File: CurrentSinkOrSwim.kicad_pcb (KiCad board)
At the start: 2 copper layers, 41.7 x 47.8 mm, 22 parts, among them P1 HEATSINK, P101 CONN_01X02, P102 CONN_01X03, P103 CONN_01X02, Q401 BUK9575, U201 LMV358, U301 LM2931

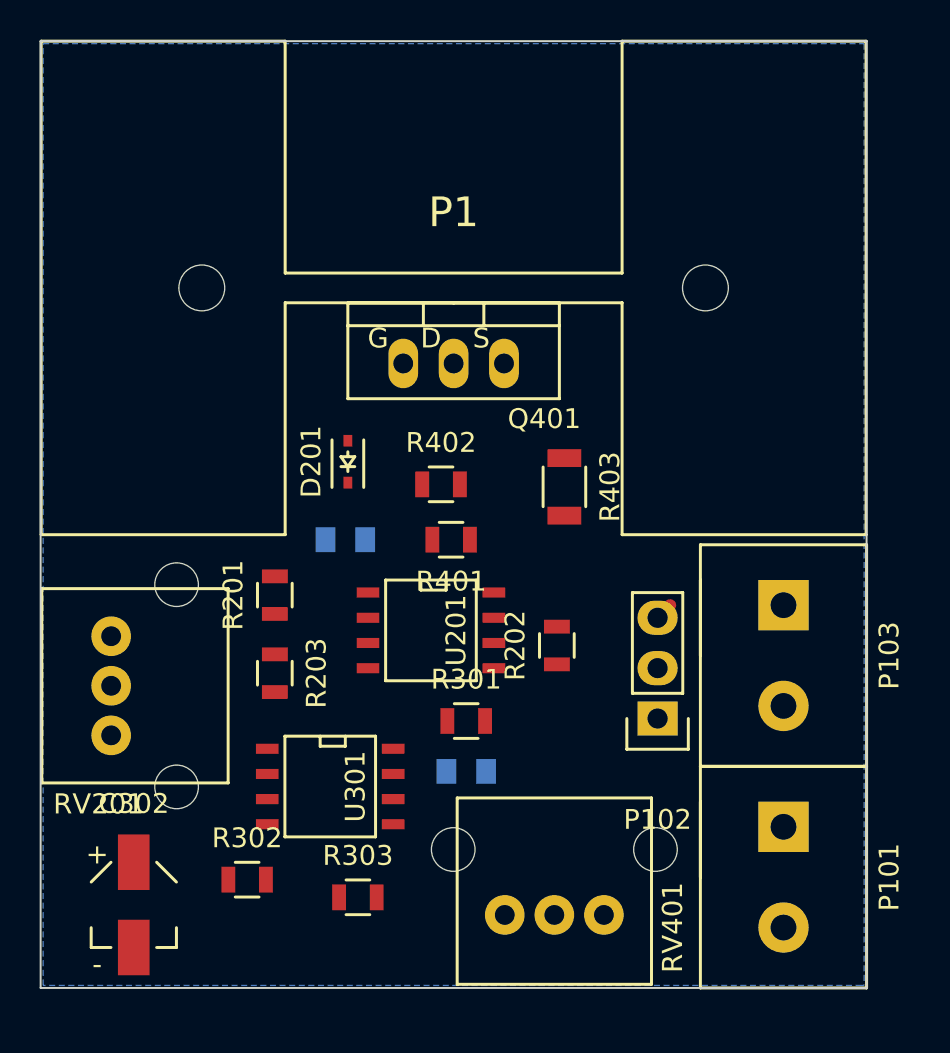
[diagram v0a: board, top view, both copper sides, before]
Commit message: possible layout with over half of tracks
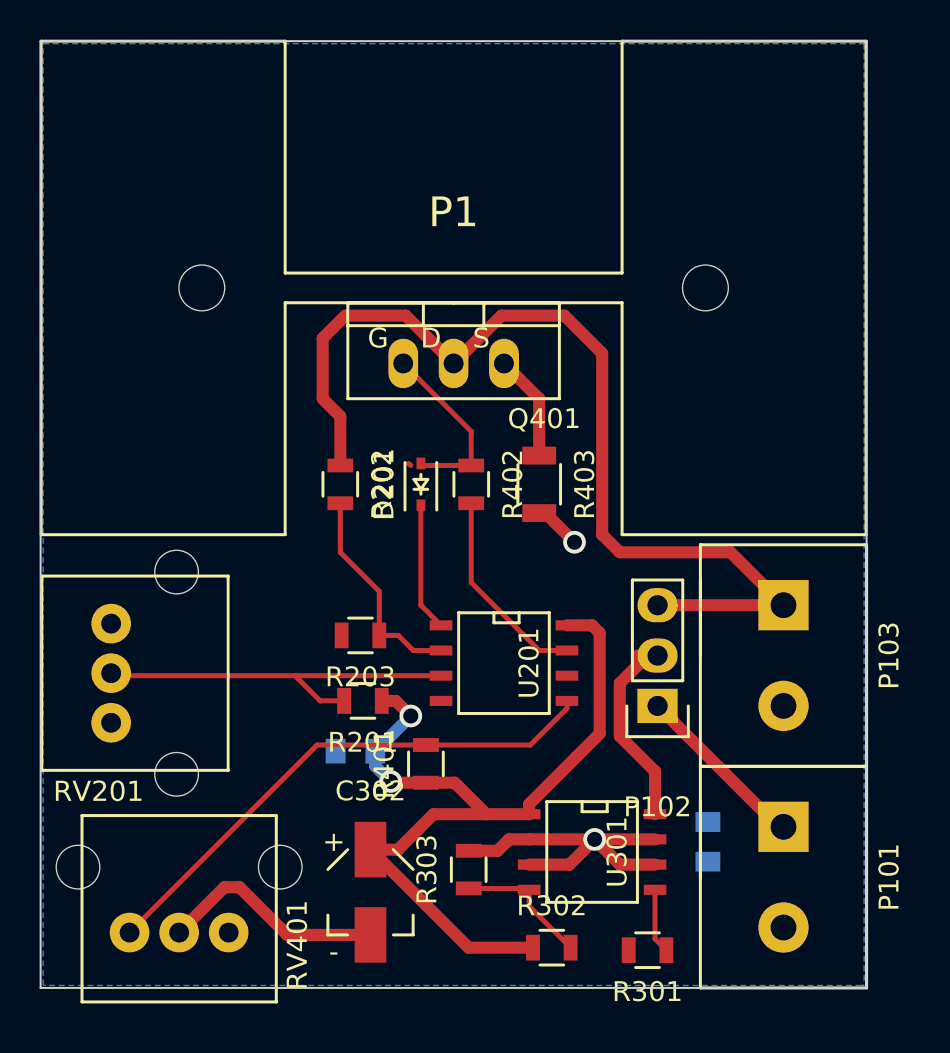
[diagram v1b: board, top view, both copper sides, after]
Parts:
- moved RV401 18.9 mm to (113.2, 80.8)
- moved R302 15.7 mm to (132.0, 81.5)
- moved R301 14.7 mm to (136.8, 81.7), turned to 180 degrees
- moved U301 13.6 mm to (134.0, 76.7)
- moved R202 13.6 mm to (121.3, 58.2), turned to 270 degrees
- moved C301 12.7 mm to (139.8, 76.2), turned to 270 degrees
- moved C302 12.0 mm to (122.8, 78.7)
- moved R401 11.4 mm to (125.6, 72.3), turned to 90 degrees
- moved C201 10.7 mm to (122.0, 71.6), turned to 180 degrees
- moved R201 6.94 mm to (122.4, 69.1), turned to 180 degrees
- moved R303 5.76 mm to (127.8, 77.6), turned to 90 degrees
- moved R203 4.72 mm to (122.3, 65.8), turned to 180 degrees
- moved U201 4.04 mm to (129.5, 67.2)
- moved D201 3.86 mm to (125.3, 58.2)
- moved R402 1.52 mm to (127.9, 58.2), turned to 270 degrees
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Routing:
- net /Current Control/Current_Sink+: track 1.66 -> 50.3 mm
- net 2.7V: track 0.00 -> 43.1 mm, vias 0 -> 2
- net GND: track 0.00 -> 31.1 mm, vias 0 -> 2
- net Net-(R401-Pad2): track 0.00 -> 27.2 mm
- net Net-(R201-Pad2): track 0.00 -> 19.7 mm
- net Net-(R202-Pad2): track 0.00 -> 10.9 mm
- net /Power Regulation/Vin: track 0.00 -> 10.8 mm
- net Net-(R402-Pad2): track 0.00 -> 10.2 mm
- net /Current Control/FET_Gate: track 0.00 -> 9.69 mm
- net Net-(P101-Pad1): track 0.00 -> 8.88 mm
- net Net-(R302-Pad2): track 0.00 -> 6.86 mm
- net Net-(D201-Pad1): track 0.00 -> 6.48 mm
- net Net-(Q401-PadS): track 0.00 -> 5.38 mm
- net Net-(R301-Pad1): track 0.00 -> 3.28 mm
